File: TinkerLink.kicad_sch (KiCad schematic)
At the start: 20 parts, among them J1 Conn_01x06_Pin, Q1 IRF4905S, Q2 MMBT2222A, SW1 TS-061D-250D4-P, U1 ESP-01F-2M, U2 ME6211C33M5

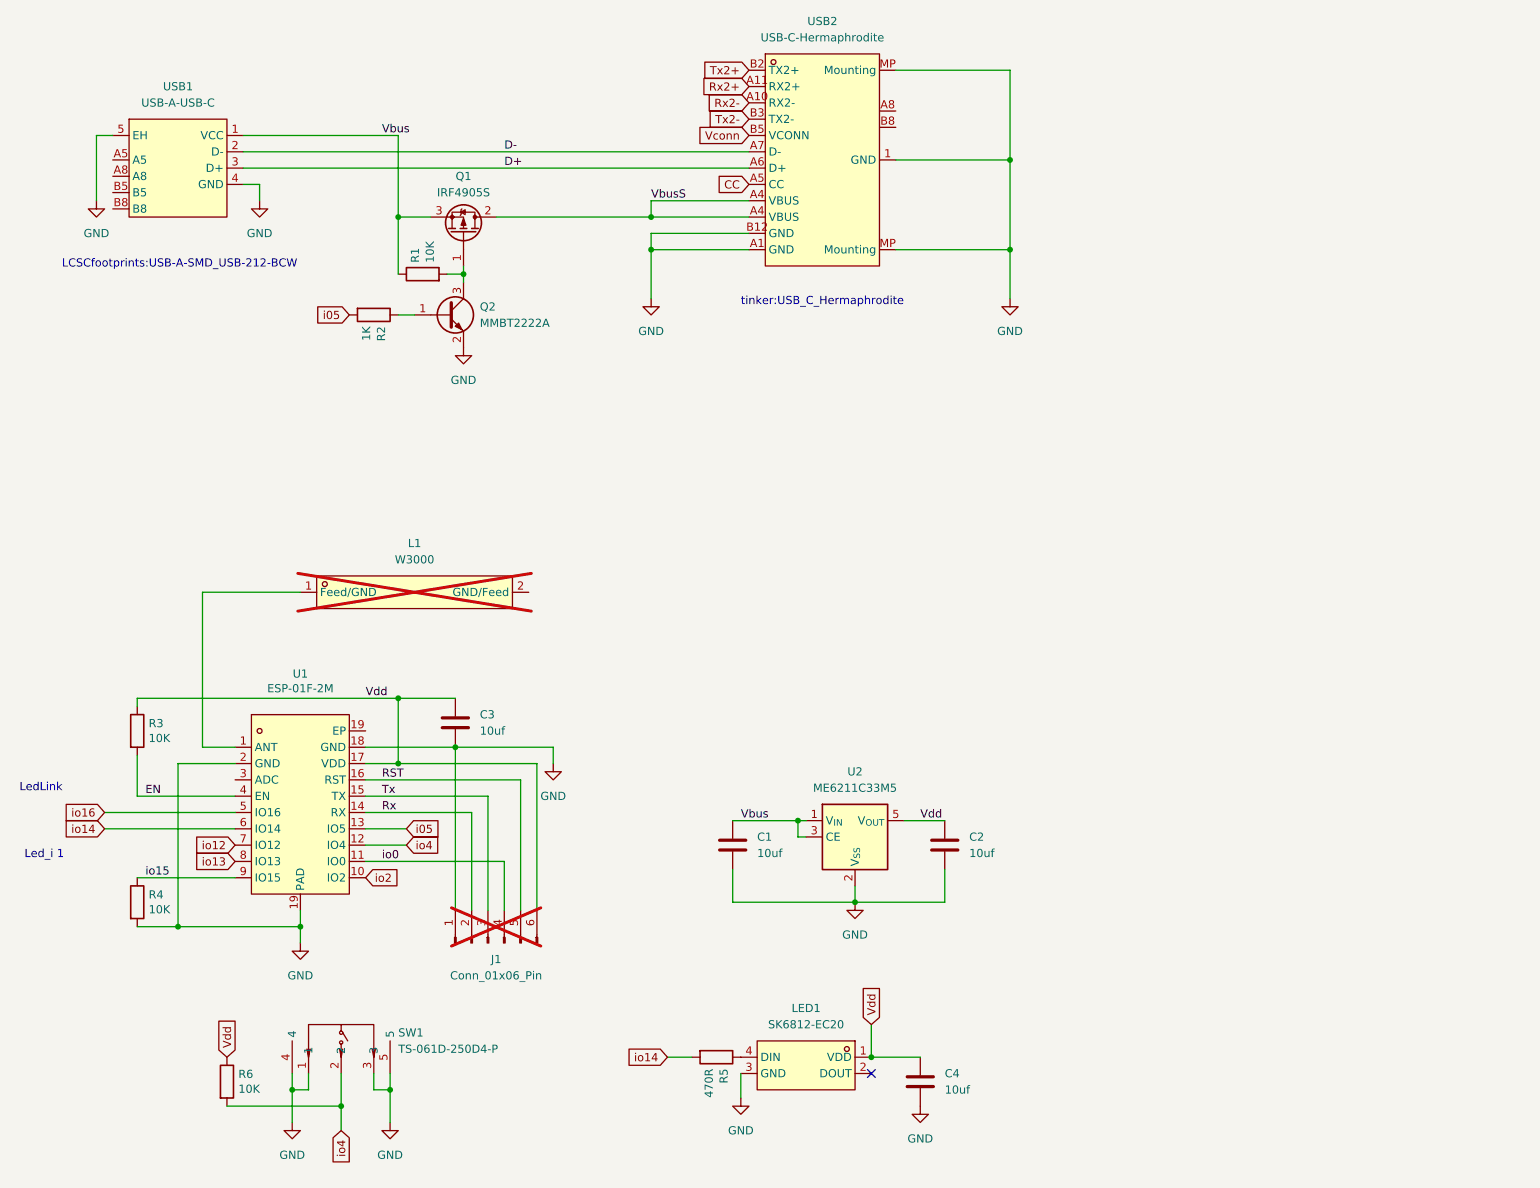
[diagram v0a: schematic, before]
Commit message: aaannnddd tweakin'...
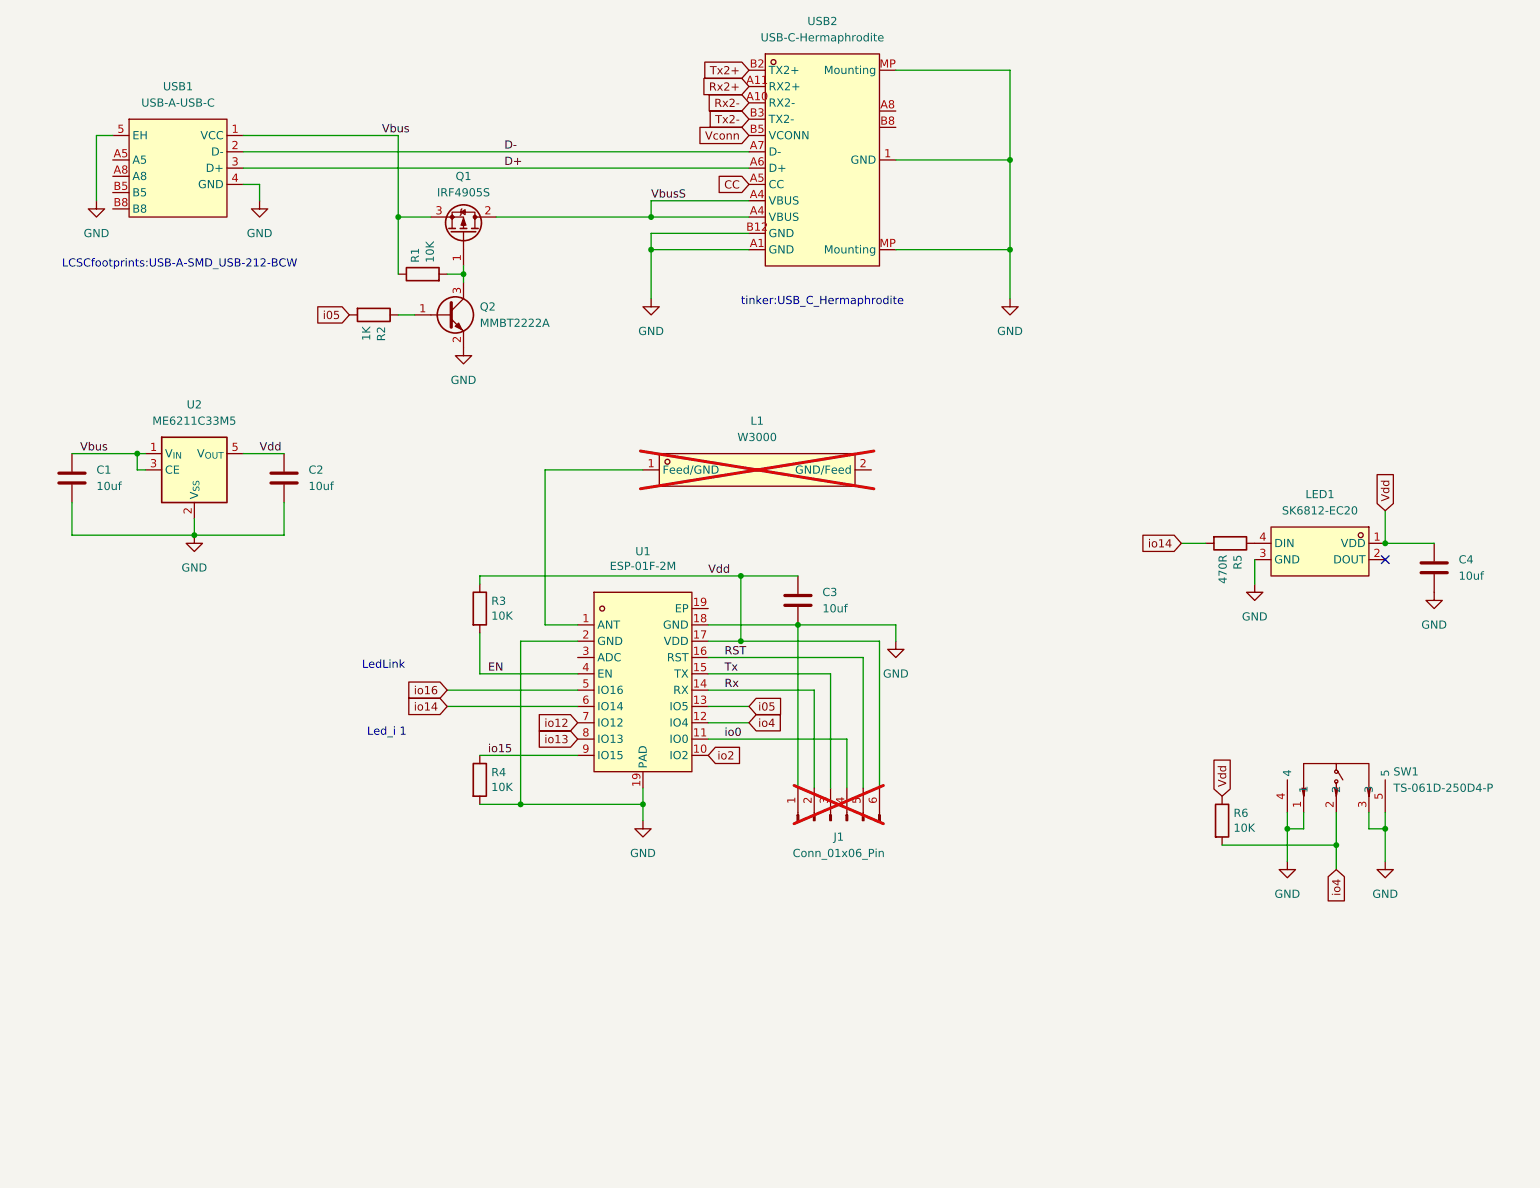
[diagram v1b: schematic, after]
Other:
- title: (none) -> TinkerLink
- moved on the sheet: C1, C2, C3, C4, J1, L1, LED1, R3, R4, R5, R6, SW1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
